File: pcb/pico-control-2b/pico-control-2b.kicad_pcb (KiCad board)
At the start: 2 copper layers, 33.1 x 65.8 mm, 26 parts, among them J1 Conn_01x07_Pin, J2 Conn_01x08_Socket, J4 Conn_01x02_Socket, SW1 SW_Push, SW2 SW_DIP_x02, U1 Pico

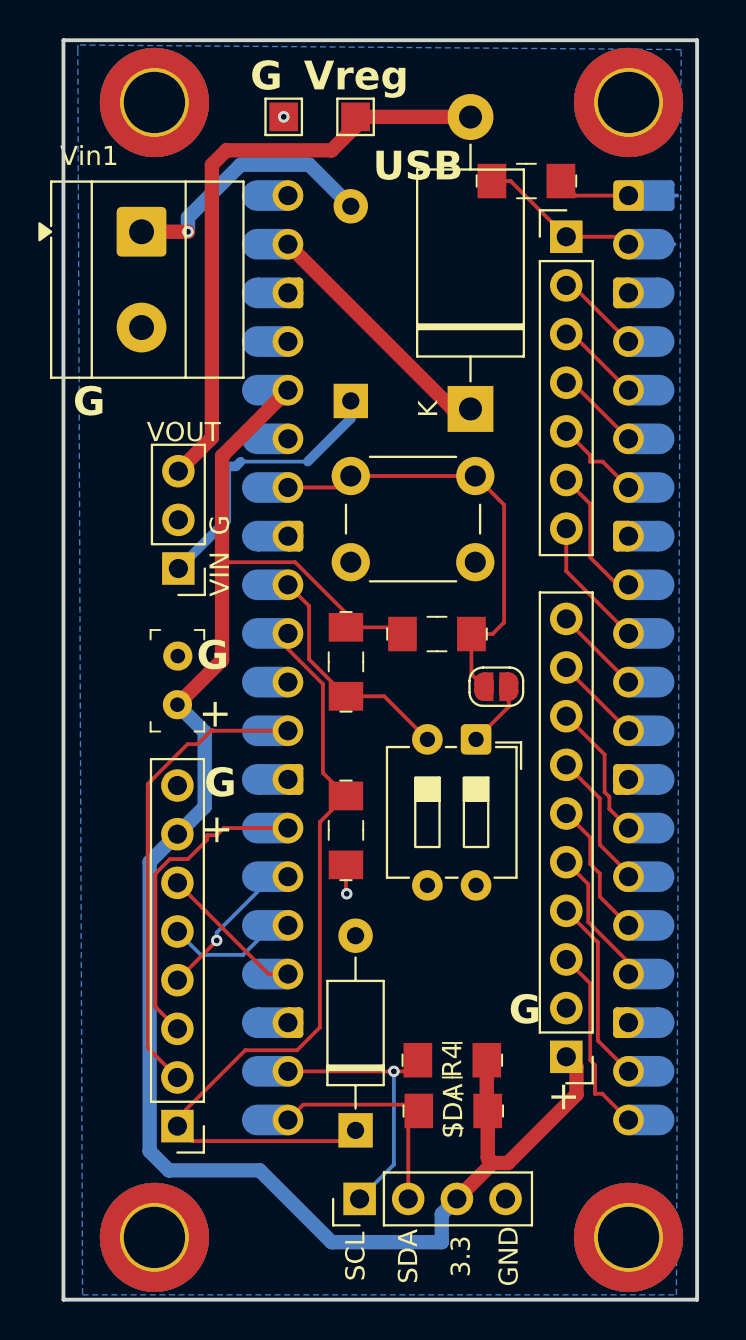
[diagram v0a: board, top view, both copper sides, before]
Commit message: PCB fixes and adjustments
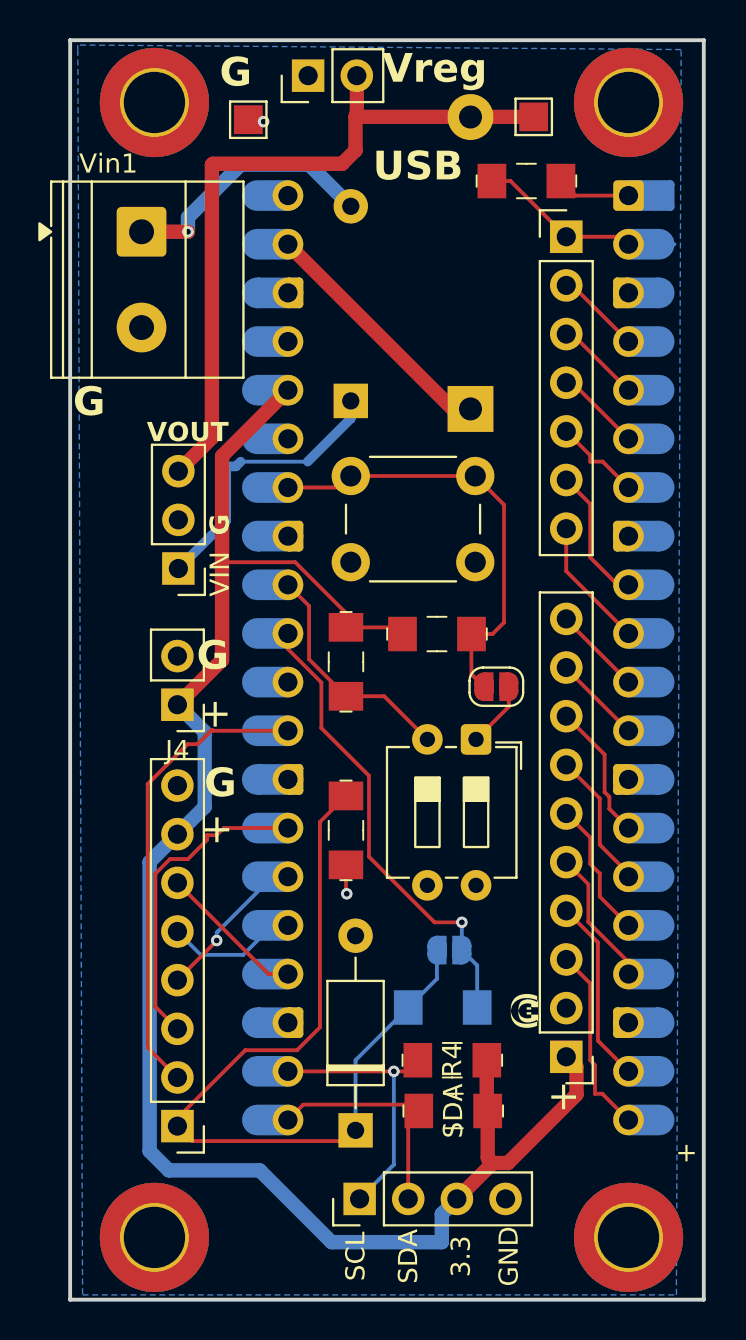
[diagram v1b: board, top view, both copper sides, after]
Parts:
- added J5: Conn_01x02_Socket, Connector_PinHeader_2.54mm:PinHeader_1x02_P2.54mm_Vertical, F.Cu at (143.0, 58.6)
- added JP2: SolderJumper_2_Open, Jumper:SolderJumper-2_P1.3mm_Open_RoundedPad1.0x1.5mm, B.Cu at (150.4, 104.2)
- added R5: R, digikey-footprints:1206, B.Cu at (150.1, 107.2)
- D1: moved to B.Cu
- J4: footprint digikey-footprints:PinHeader_1x2_P2.54mm -> Connector_PinHeader_2.54mm:PinHeader_1x02_P2.54mm_Vertical
- moved VREG2 9.30 mm to (154.8, 60.8)
- moved G1 1.86 mm to (139.9, 60.9)
- turned J4 to 180 degrees
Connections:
- U1 pad 31: Net-(D4-K) -> Net-(JP2-B)
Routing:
- net Net-(JP2-B): track 0.00 -> 24.5 mm, vias 0 -> 1
- net +5V: track 31.6 -> 37.8 mm
- net Net-(U1-GPIO0): track 5.58 -> 3.84 mm
- net Net-(D4-K): track 42.1 -> 43.6 mm
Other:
- board text added: "A Sel"
